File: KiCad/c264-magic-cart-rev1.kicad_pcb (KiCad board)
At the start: 2 copper layers, 56 x 91 mm, 10 parts, among them IC1 27C080, IC2 74LS/HCT273, IC3 27C160, IC5 GAL20V8

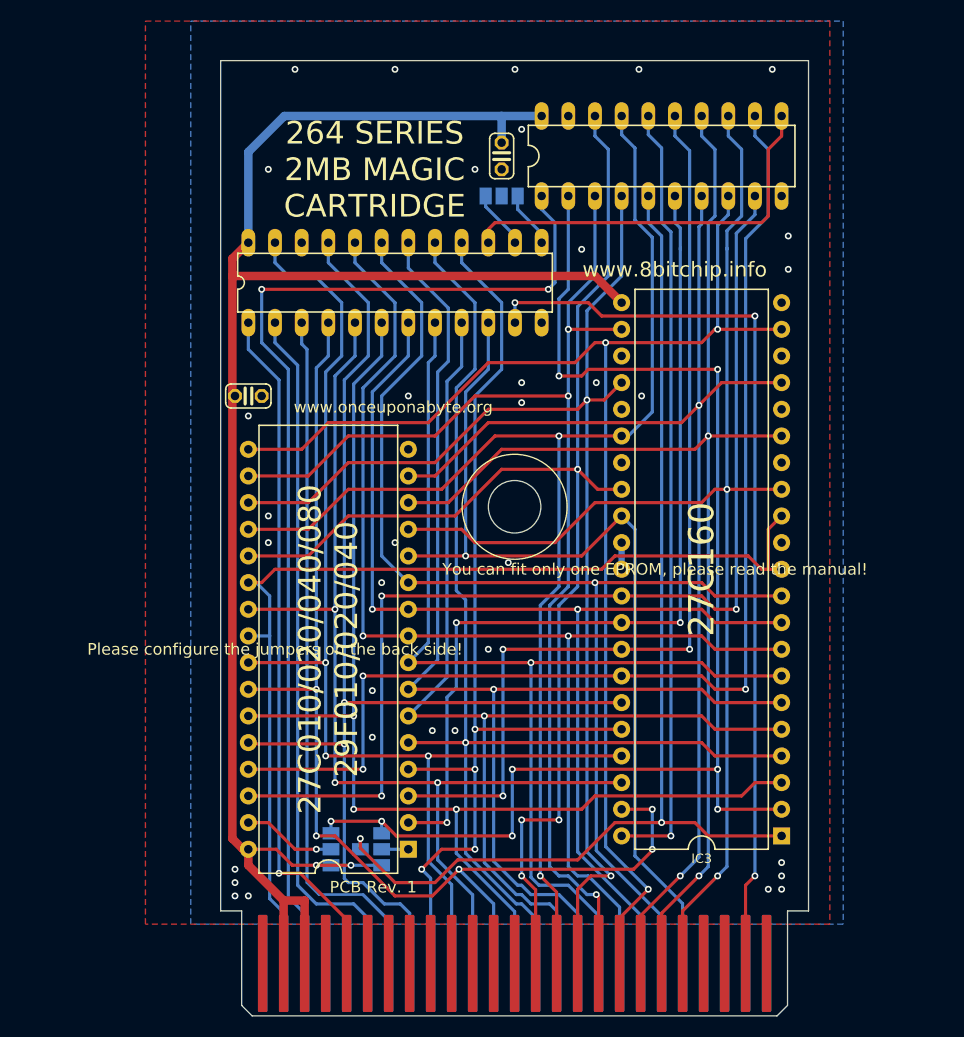
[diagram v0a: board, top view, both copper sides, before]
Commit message: Some rought edges, but ready for V1S
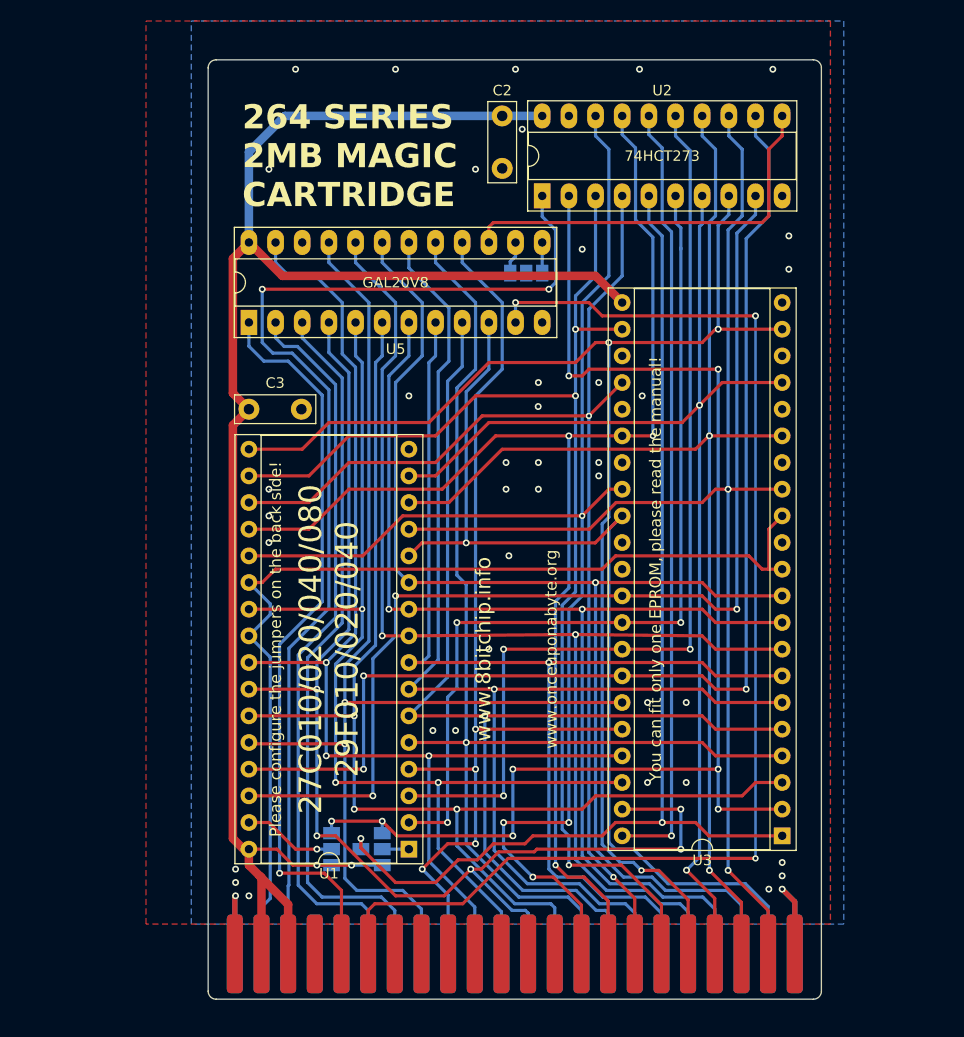
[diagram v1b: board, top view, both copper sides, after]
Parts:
- removed IC1: 27C080, c264-magic-cart-rev1:DIL32
- removed U$1: C16_CARTRIDGE, c264-magic-cart-rev1:C16_CART
- added CN1: C16_NEWSTYLE_EXP_PORT, c264-magic-cart-rev1:EdgeConn-44pin, F.Cu at (148.5, 148.8)
- added U1: 27C080, Package_DIP:DIP-32_W15.24mm_Socket, F.Cu at (138.4, 134.6)
- C2, C3: value (none) -> 100n; footprint c264-magic-cart-rev1:C025-024X044_334 -> Capacitor_THT:C_Disc_D7.5mm_W2.5mm_P5.00mm
- CONFIG0: value (none) -> SJ2W; footprint c264-magic-cart-rev1:SJ_2_252 -> c264-magic-cart-rev1:SJ_2
- SJ1: value (none) -> SJ2W
- U2: renamed from IC2; value 74LS/HCT273 -> 74HCT273; footprint c264-magic-cart-rev1:DIL20_85 -> Package_DIP:DIP-20_W7.62mm_Socket_LongPads
- U3: renamed from IC3; footprint c264-magic-cart-rev1:DIP42 -> Package_DIP:DIP-42_W15.24mm_Socket
- U5: renamed from IC5; footprint c264-magic-cart-rev1:DIL24-3_321 -> Package_DIP:DIP-24_W7.62mm_Socket_LongPads
- moved U3 26.5 mm to (174.0, 133.3), turned to 180 degrees
- moved U5 14.4 mm to (123.2, 84.4), turned to 90 degrees
- moved U2 12.0 mm to (151.1, 72.4), turned to 90 degrees
- moved CONFIG0 7.71 mm to (149.6, 79.7)
- moved C2 3.82 mm to (147.3, 64.8)
- moved C3 1.26 mm to (123.2, 92.7)
- moved SJ1 0.05 mm to (131.1, 134.6)
- moved U$2 0.05 mm to (135.9, 134.6)
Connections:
- net /CRT renamed //CRT
- net A0 renamed /A0
- net A1 renamed /A1
- net A10 renamed /A10
- net A11 renamed /A11
- net A12 renamed /A12
- net A13 renamed /A13
- net A2 renamed /A2
- net A3 renamed /A3
- net A4 renamed /A4
- net A5 renamed /A5
- net A6 renamed /A6
- net A7 renamed /A7
- net A8 renamed /A8
- net A9 renamed /A9
- net AA14 renamed /AA14
- net AA15 renamed /AA15
- net AA16 renamed /AA16
- net AA17 renamed /AA17
- net AA18 renamed /AA18
- net AA19 renamed /AA19
- net AA20 renamed /AA20
- net AA21 renamed /AA21
- net C1LO renamed /C1LO
- net CFG0 renamed /CFG0
- net CFG1 renamed /CFG1
- net D0 renamed /D0
- net D1 renamed /D1
- net D2 renamed /D2
- net D3 renamed /D3
- net D4 renamed /D4
- net D5 renamed /D5
- net D6 renamed /D6
- net D7 renamed /D7
- SJ1 pad 2: PIN31 -> /PIN31
- U$2 pad 2: PIN1 -> /PIN1
- U2 pad 1: /RESET -> //RESET
- U3 pad 15: (no net) -> unconnected-(U3-Q8-Pad15)
- U3 pad 17: (no net) -> unconnected-(U3-Q9-Pad17)
- U3 pad 19: (no net) -> unconnected-(U3-Q10-Pad19)
- U3 pad 21: (no net) -> unconnected-(U3-Q11-Pad21)
- U3 pad 24: (no net) -> unconnected-(U3-Q12-Pad24)
- U3 pad 26: (no net) -> unconnected-(U3-Q13-Pad26)
- U3 pad 28: (no net) -> unconnected-(U3-Q14-Pad28)
- U5 pad 1: R/W -> /R/W
- U5 pad 11: PHI2 -> /PHI2
- U5 pad 2: A15 -> /A15
- U5 pad 22: (no net) -> unconnected-(U5-IO22-Pad22)
- U5 pad 3: A14 -> /A14
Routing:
- net /PHI2: track 0.00 -> 120.1 mm, vias 0 -> 3
- net //RESET: track 0.00 -> 105.6 mm, vias 0 -> 2
- net /RESET: track 102.9 -> 0.00 mm, vias 2 -> 0
- net PHI2: track 87.3 -> 0.00 mm, vias 3 -> 0
- net /R/W: track 0.00 -> 71.0 mm, vias 0 -> 1
- net /A15: track 0.00 -> 70.0 mm
- net /A14: track 0.00 -> 69.8 mm
- net A14: track 66.9 -> 0.00 mm
- net A15: track 66.8 -> 0.00 mm
- net R/W: track 66.1 -> 0.00 mm, vias 1 -> 0
- net GND: track 2.54 -> 24.4 mm, vias 35 -> 41
- net PIN31: track 8.93 -> 0.00 mm, vias 1 -> 0
- net /PIN31: track 0.00 -> 8.93 mm, vias 0 -> 1
- net /A0: track 90.0 -> 97.6 mm
- net /A9: track 109.2 -> 116.8 mm
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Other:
- board size 56 x 91 mm -> 58.4 x 89.5 mm
- board text added: "CONFIG"
- board text added: "Hardware Design: Marko Šolajić 44-Pin Version: SukkoPera Generator Software: Žarko Živanov"
- board text added: "V1S"
- board text removed: "Hardware design: Marko Šolajić Generator Software: Žarko Živanov"
- board text removed: "PCB Rev. 1"
